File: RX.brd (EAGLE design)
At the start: 50 x 50 mm, 41 parts, among them IC1 MEGA8-AI, IC2 LM358D, Q1 16M

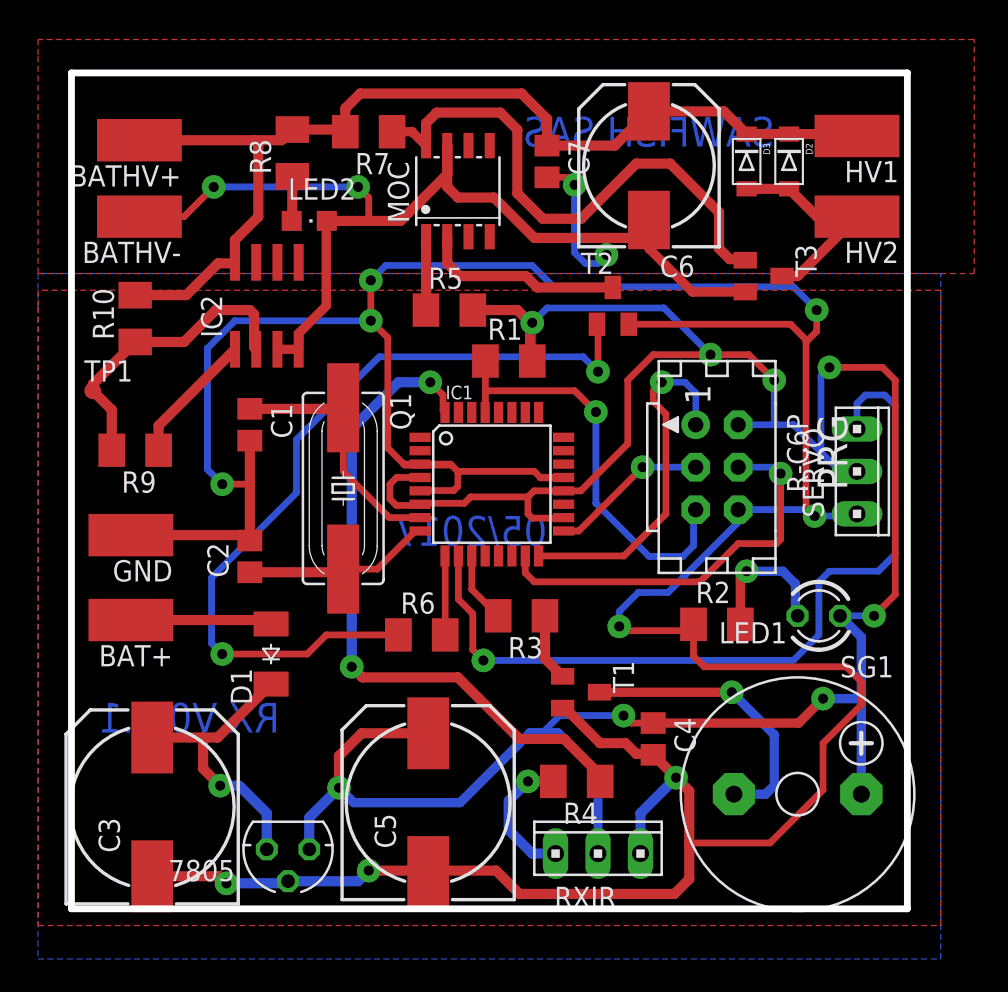
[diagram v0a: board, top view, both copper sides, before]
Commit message: 21/06/2017
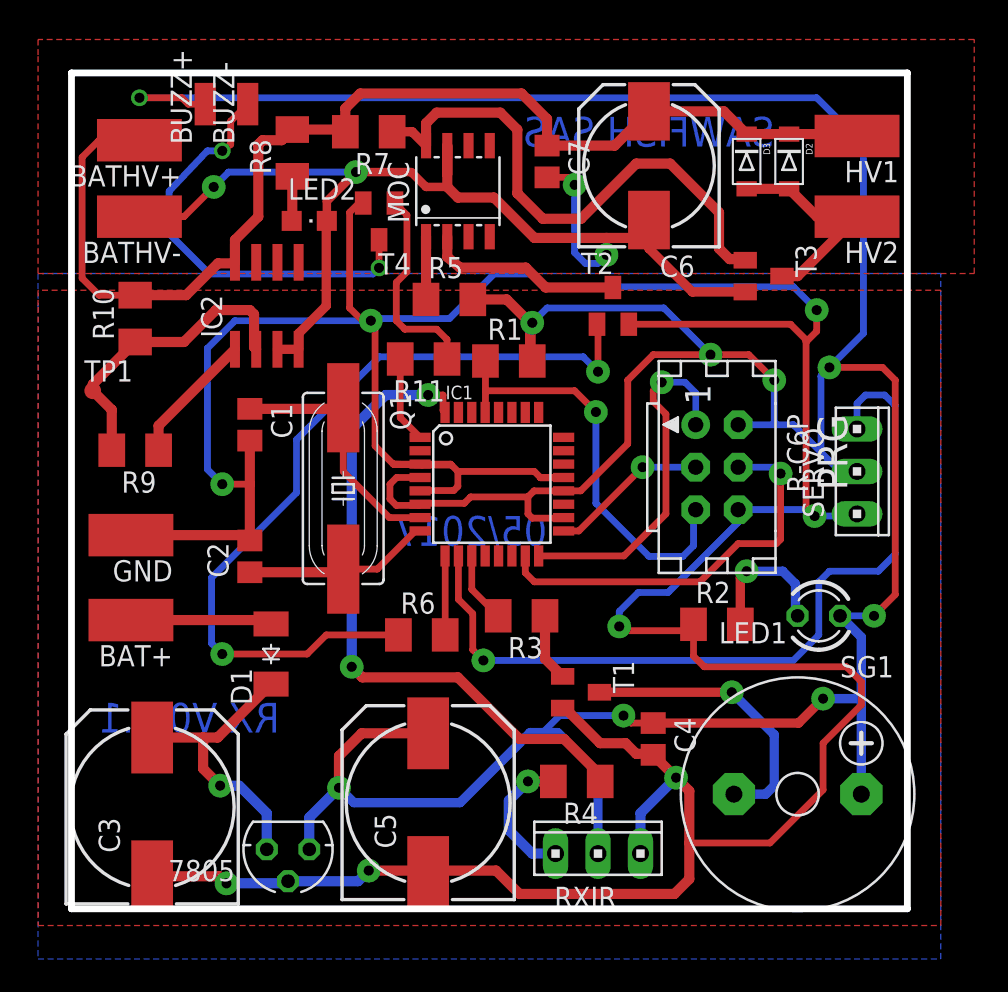
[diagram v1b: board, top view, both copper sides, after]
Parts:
- added BUZZ+, BUZZ-: (no value), wirepad:SMD1,27-2,54
- added R11: 1k, rcl:M1206
- added T4: (no value), transistor-neu-to92:SOT23-BEC
- moved R5 0.63 mm to (22.6, 36.4)
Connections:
- new net N$17: IC1.1, R11.2
- new net N$18: BUZZ-.1, T4.C
- new net N$4: R11.1, T4.B
- net +5V: now also BUZZ+.1
- net GND: now also T4.E
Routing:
- net +5V: track 160.8 -> 223.8 mm, vias 8 -> 9
- net N$18: track 0.00 -> 25.6 mm, vias 0 -> 2
- net N$4: track 0.00 -> 12.3 mm
- net GND: track 221.5 -> 228.9 mm, vias 9 -> 8
- net VCC: track 63.5 -> 70.8 mm
- net N$17: track 0.00 -> 5.18 mm
- net AGND: track 69.9 -> 69.0 mm
- net N$10: track 4.39 -> 3.75 mm
- net RXIR: track 40.2 -> 39.5 mm
